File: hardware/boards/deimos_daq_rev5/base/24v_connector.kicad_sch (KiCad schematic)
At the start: 16 parts, among them IC8001 INA826AIDR, J8001 Barrel_Jack PJ-202BH, U4001 INA181A2

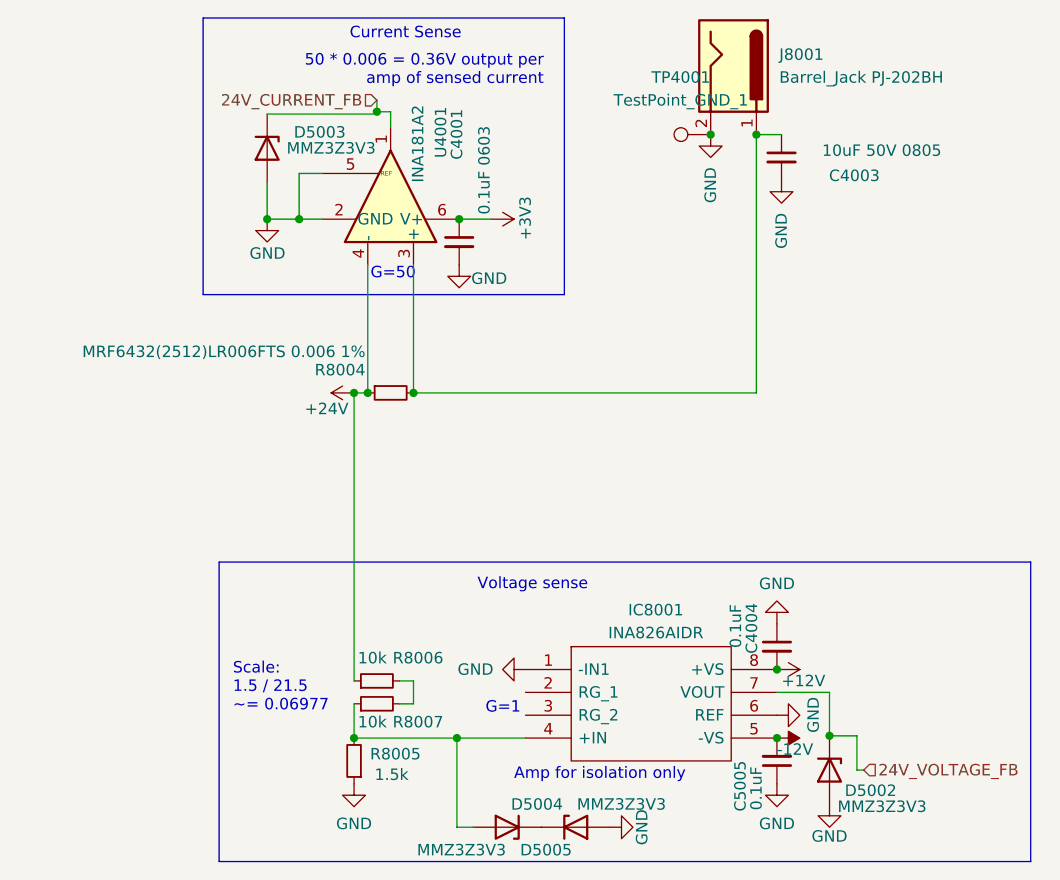
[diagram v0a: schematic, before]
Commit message: restore rev5 and make this rev rev6
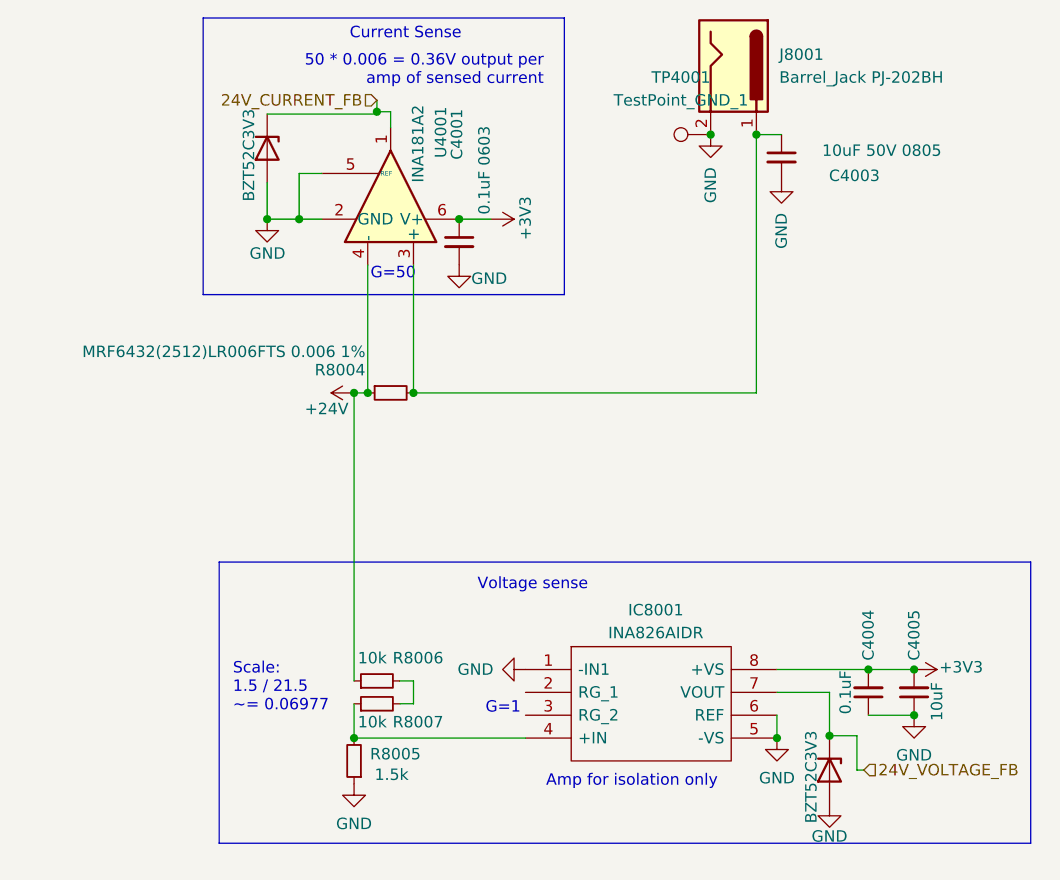
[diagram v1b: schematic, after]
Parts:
- removed C5005: 0.1uF, Capacitor_SMD:C_0402_1005Metric, symbol Device:C_Small
- removed D5004, D5005: MMZ3Z3V3, Diode_SMD:D_SOD-323, symbol Device:D_Zener
- added C4005: 10uF, Capacitor_SMD:C_0603_1608Metric, symbol Device:C_Small
- D5002, D5003: value MMZ3Z3V3 -> BZT52C3V3; LCSC C52056 -> C2112
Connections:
- net +12V is gone; now on net +3V3: C4004.2, IC8001.8 (+VS)
- net -12V is gone; now on net GND: IC8001.5 (-VS)
- net +3V3: now also C4005.2
- net GND: now also C4005.1
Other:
- moved on the sheet: C4004
